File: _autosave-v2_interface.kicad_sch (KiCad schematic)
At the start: 46 parts, among them J10 Power, J11 Vref_Select, J12 AUX_Select, J8 DE9_Socket, J9 DB25_Socket, Q1 2N7002K, Q2 2N7002K, U10 MCP1501-20xCH, U8 MCP4922, U9 MCP3424x-xSL

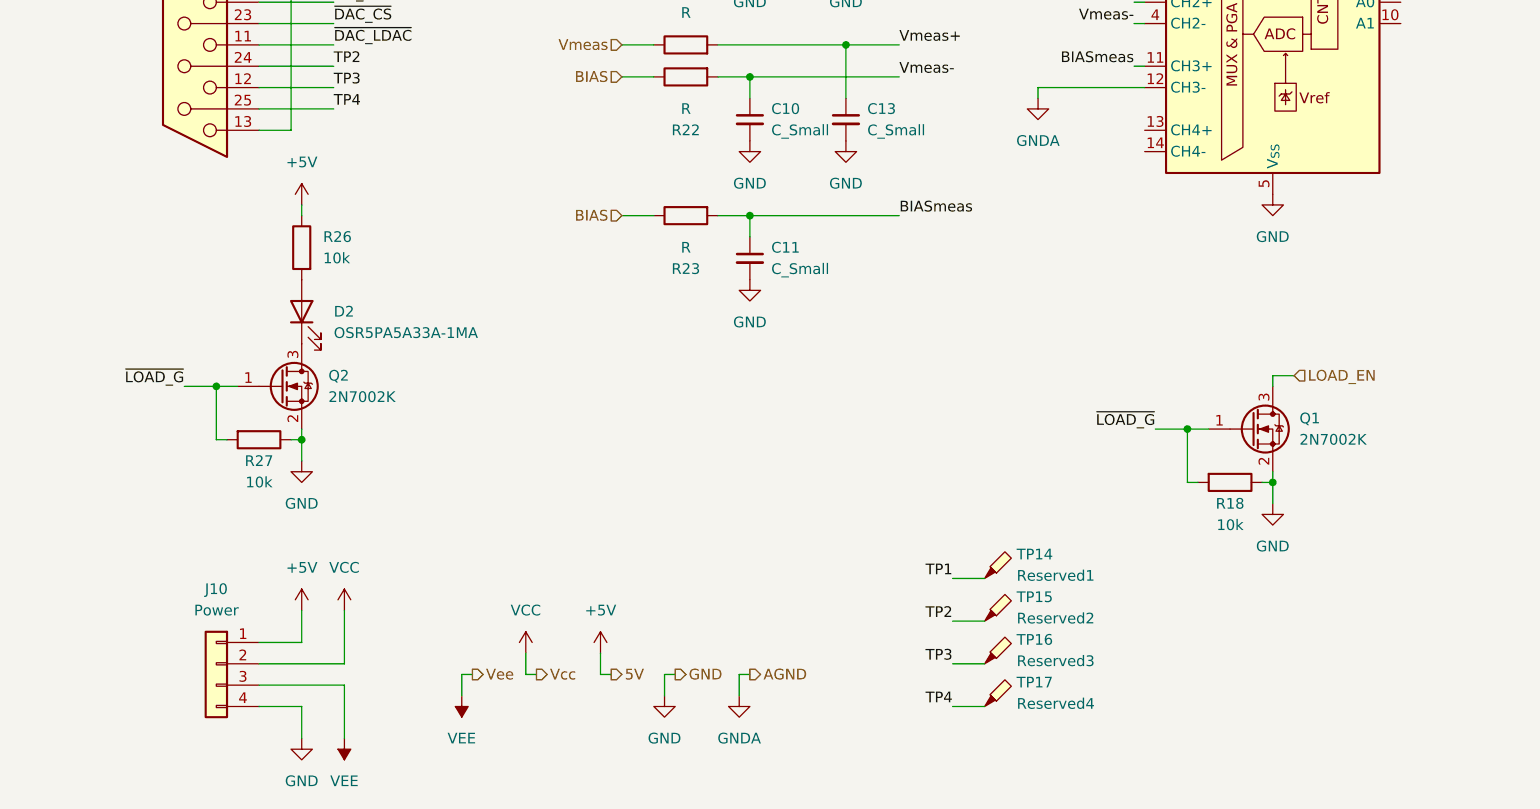
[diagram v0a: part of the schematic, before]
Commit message: おおまか
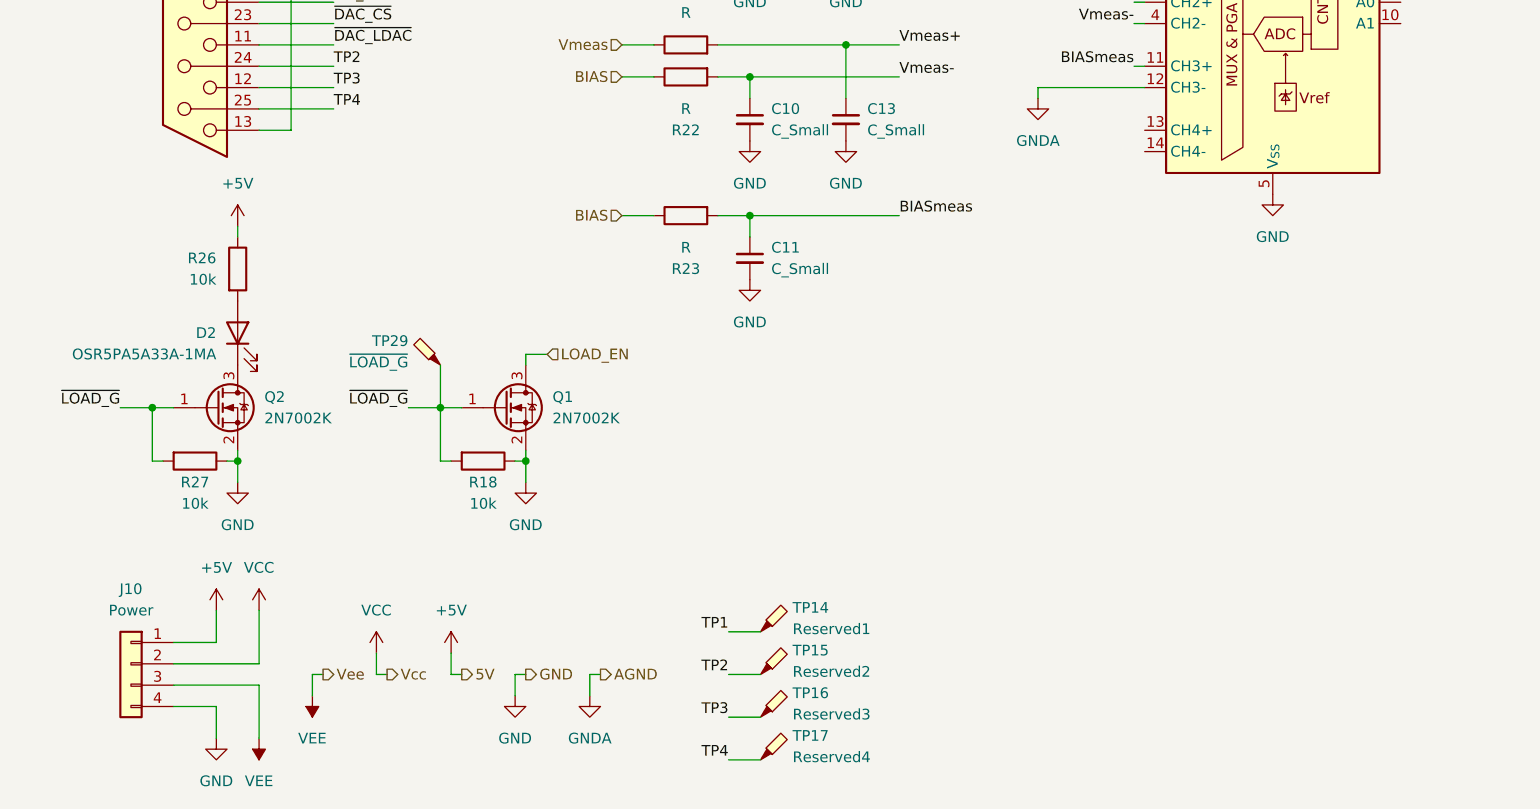
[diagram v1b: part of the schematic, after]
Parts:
- added TP29: ~{LOAD_G}, symbol Connector:TestPoint_Probe
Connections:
- net ~{LOAD_G}: now also TP29.1
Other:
- moved on the sheet: D2, J10, Q1, Q2, R18, R26, R27, TP14, TP15, TP16, TP17
